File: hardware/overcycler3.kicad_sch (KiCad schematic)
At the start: 133 parts, among them J1 USB_B, J2 AudioJack3_Switch, J3 DIN-5_180degree, J4 AudioJack3_Switch, J5 AudioJack3_Switch, P1 FT232, P2 PANEL, Q1 2SC945, SW1 RESET, SW2 POWER, U1 XT26G02CWSIGA, U2 TL064, U20 AD5328B, U3 LPC1778FBD144, U4 TLV2556, U5 74HC138, U6 TL064, U7 AD5328B, Y1 12MHz

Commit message: hardware: Schematics rework by Guimli
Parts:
- removed C10, C11, C12, C14, C15, C16, C17, C18, C19, C20, C23, C24, C25, C26, C27, C28, C29, C30, C32, C34: 100n, Capacitor_SMD:C_0805_2012Metric, symbol overcycler2-rescue:C
- removed C13: 470u, Capacitor_Tantalum_SMD:CP_EIA-7343-43_Kemet-X, symbol overcycler2-rescue:CP1
- removed C2, C3, C4, C5, C6, C7: 10n, Capacitor_SMD:C_0805_2012Metric, symbol overcycler2-rescue:C
- removed C21, C22, C31: 10u, Capacitor_Tantalum_SMD:CP_EIA-3216-18_Kemet-A, symbol overcycler2-rescue:CP1
- removed J1: USB_B, Connector_USB:USB_B_Lumberg_2411_02_Horizontal, symbol Connector:USB_B
- removed P1: FT232, Connector_PinSocket_2.54mm:PinSocket_1x06_P2.54mm_Vertical, symbol overcycler2-rescue:CONN_6
- removed P2: PANEL, Connector_IDC:IDC-Header_2x20_P2.54mm_Vertical, symbol overcycler2-rescue:CONN_20X2
- removed PS1: IA0505S-2W, JETEKPS:IA0505S-2W, symbol Converter_DCDC:IA0505S
- removed PS2: IB0503LSY-1WR1, JETEKPS:IB0503LSY, symbol Converter_DCDC:IA0503S
- removed R152: 2k7, Resistor_SMD:R_0805_2012Metric, symbol overcycler2-rescue:R
- removed R2, R4: 33, Resistor_SMD:R_0805_2012Metric, symbol overcycler2-rescue:R
- removed R5: 1k5, Resistor_SMD:R_0805_2012Metric, symbol overcycler2-rescue:R
- removed SW2: POWER, SPUN192600:SPUN192600, symbol Switch:SW_Push_DPDT
- added J10: Control_Down, Connector_JST:JST_XH_B7B-XH-A_1x07_P2.50mm_Vertical, symbol Connector_Generic:Conn_01x07
- added J6: Control_Up, Connector_JST:JST_XH_B7B-XH-A_1x07_P2.50mm_Vertical, symbol Connector_Generic:Conn_01x07
- added J7: Keyboard, Connector_JST:JST_XH_B8B-XH-A_1x08_P2.50mm_Vertical, symbol Connector_Generic:Conn_01x08
- added J8: Display, Connector_IDC:IDC-Header_2x08_P2.54mm_Vertical, symbol Connector_Generic:Conn_02x08_Odd_Even
- added J9: FT232, Connector_PinSocket_2.54mm:PinSocket_1x06_P2.54mm_Vertical, symbol Connector_Generic:Conn_01x06
- C1, C112, C113, C114, C35, C37, C38, C39, C40, C41, C42, C43, C44, C45, C46, C47, C50, C51, C8, C9: symbol overcycler2-rescue:C -> Additional:C
- C33, C36, C48, C49: symbol overcycler2-rescue:CP1 -> Additional:CP
- D1, D2, D3, D4, D5: symbol overcycler2-rescue:DIODE -> Additional:DIODE
- OC1: symbol overcycler2-rescue:6N139 -> Isolator:6N139
- R1, R10, R11, R12, R13, R14, R15, R16, R17, R18, R19, R20, R21, R22, R23, R24, R25, R26, R27, R28, R29, R3, R30, R31, R32, R33, R34, R35, R36, R37, R38, R39, R40, R45, R46, R47, R48, R6, R7, R8, R9: symbol overcycler2-rescue:R -> Additional:R
- R151, R41, R42, R43, R44: renamed from R93; symbol overcycler2-rescue:R -> Additional:R
- SW1: symbol overcycler2-rescue:SW_PUSH -> Additional:SW_PUSH
- U1: symbol XT26G02ELGIGA:XT26G02ELGIGA -> Additional:XT26G02ELGIGA
- U2, U6: symbol overcycler2-rescue:TL074 -> Amplifier_Operational:TL064
- U20, U7: symbol AD5328B:AD5328B -> Additional:AD5328B
- U3: symbol LPC1778FBD144:LPC1778FBD144 -> Additional:LPC1778FBD144; Supplier C37701 -> (none)
- U4: symbol overcycler2-rescue:TLV1543 -> Additional:TLV1543
- U5: symbol overcycler2-rescue:74LS138 -> 74xx:74HC138
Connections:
- net +5V: now also U20.1 (~{LDAC}), U7.1 (~{LDAC}), J8.14 (Pin_14); no longer U2.4 (V+), U2.4 (V+), U2.4 (V+), U2.4 (V+), U6.4 (V+), U6.4 (V+), U6.4 (V+), U6.4 (V+)
- net -5V: no longer U2.11 (V-), U2.11 (V-), U2.11 (V-), U2.11 (V-), U6.11 (V-), U6.11 (V-), U6.11 (V-), U6.11 (V-)
- net GND: now also U1.9 (PAD), J10.7 (Pin_7), J6.7 (Pin_7), J8.13 (Pin_13), J9.4 (Pin_4); no longer U20.1 (/LDAC), U7.1 (/LDAC)
- net KP_1_R1: now also J7.1 (Pin_1)
- net KP_2_R2: now also J7.2 (Pin_2)
- net KP_3_R3: now also J7.3 (Pin_3)
- net KP_4_R4: now also J7.4 (Pin_4)
- net KP_5_C1: now also J7.5 (Pin_5)
- net KP_6_C2: now also J7.6 (Pin_6)
- net KP_7_C3: now also J7.7 (Pin_7)
- net KP_8_C4: now also J7.8 (Pin_8)
- net LCD_CTRST: now also R25.1, J8.12 (Pin_12); no longer R25.2, U3.8 (P0[26])
- net LCD_DB4: now also J8.4 (Pin_4)
- net LCD_DB5: now also J8.3 (Pin_3)
- net LCD_DB6: now also J8.2 (Pin_2)
- net LCD_DB7: now also J8.1 (Pin_1)
- net LCD_E1: now also J8.9 (Pin_9)
- net LCD_E2: now also J8.15 (Pin_15)
- net LCD_RS: now also J8.11 (Pin_11)
- net LCD_RW: now also J8.10 (Pin_10)
- net PROG_BOOT: now also J9.6 (Pin_6)
- net PROG_RXD: now also J9.3 (Pin_3)
- net PROG_TXD: now also J9.2 (Pin_2)
- net P_0: now also J6.2 (Pin_2)
- net P_1: now also J6.3 (Pin_3)
- net P_2: now also J6.4 (Pin_4)
- net P_3: now also J6.5 (Pin_5)
- net P_4: now also J6.6 (Pin_6)
- net P_5: now also J10.2 (Pin_2)
- net P_6: now also J10.3 (Pin_3)
- net P_7: now also J10.4 (Pin_4)
- net P_8: now also J10.5 (Pin_5)
- net P_9: now also J10.6 (Pin_6)
- net SPI_SSEL: now also U5.6 (E2); no longer U5.4 (E1)
- net +3.3V renamed +3V3
- net +3V3: now also U5.4 (~{E0}), J10.1 (Pin_1), J6.1 (Pin_1), J9.1 (Pin_1); no longer U5.6 (E3)
- new net: R25.2, U3.8 (P0[26])
- no-connect marks 0 -> 96
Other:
- added sheet Power_Supply (Power_Supply.kicad_sch)
- note removed: "LCD Display is NHD‐0440WH Keypad is 16 keys 4*4 matrix Data entry potentiometers are 4.7k linear taper"
- moved on the sheet: C1, C112, C113, C114, C33, C35, C36, C37, C38, C39, C40, C41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

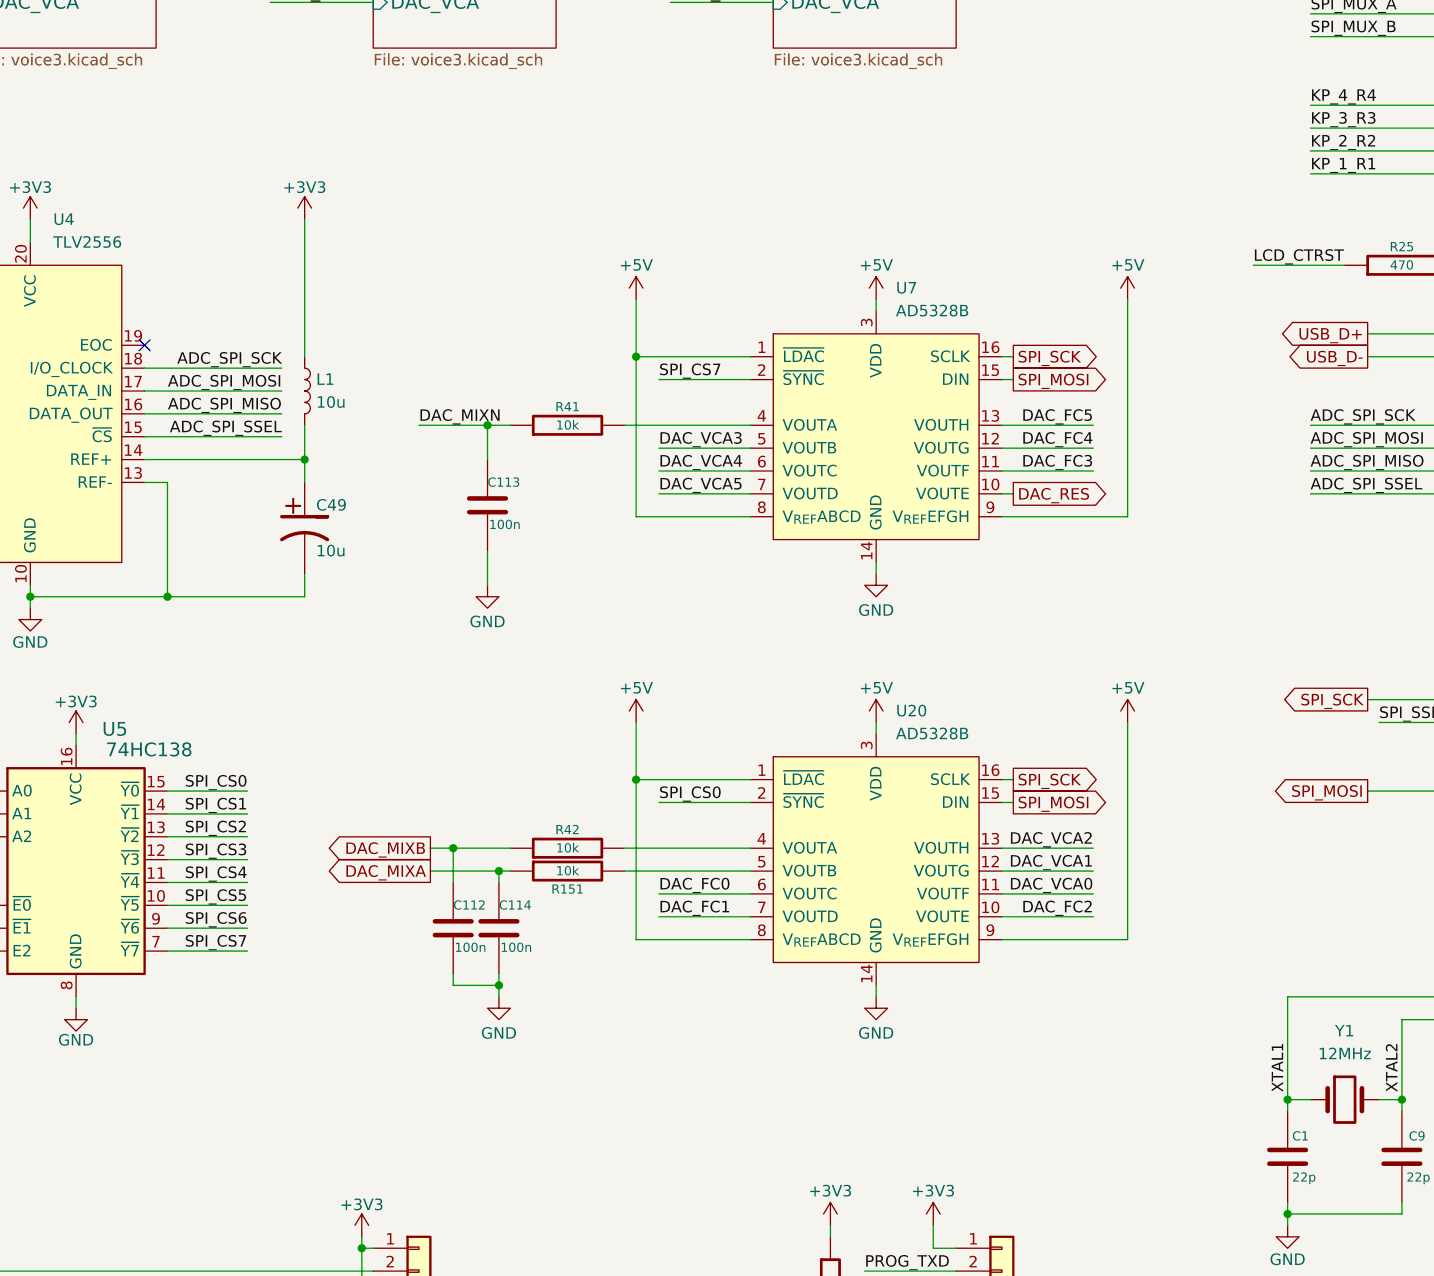
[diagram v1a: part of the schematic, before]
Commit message: hardware: sch update (AD5674R replacing AD5328B*2)
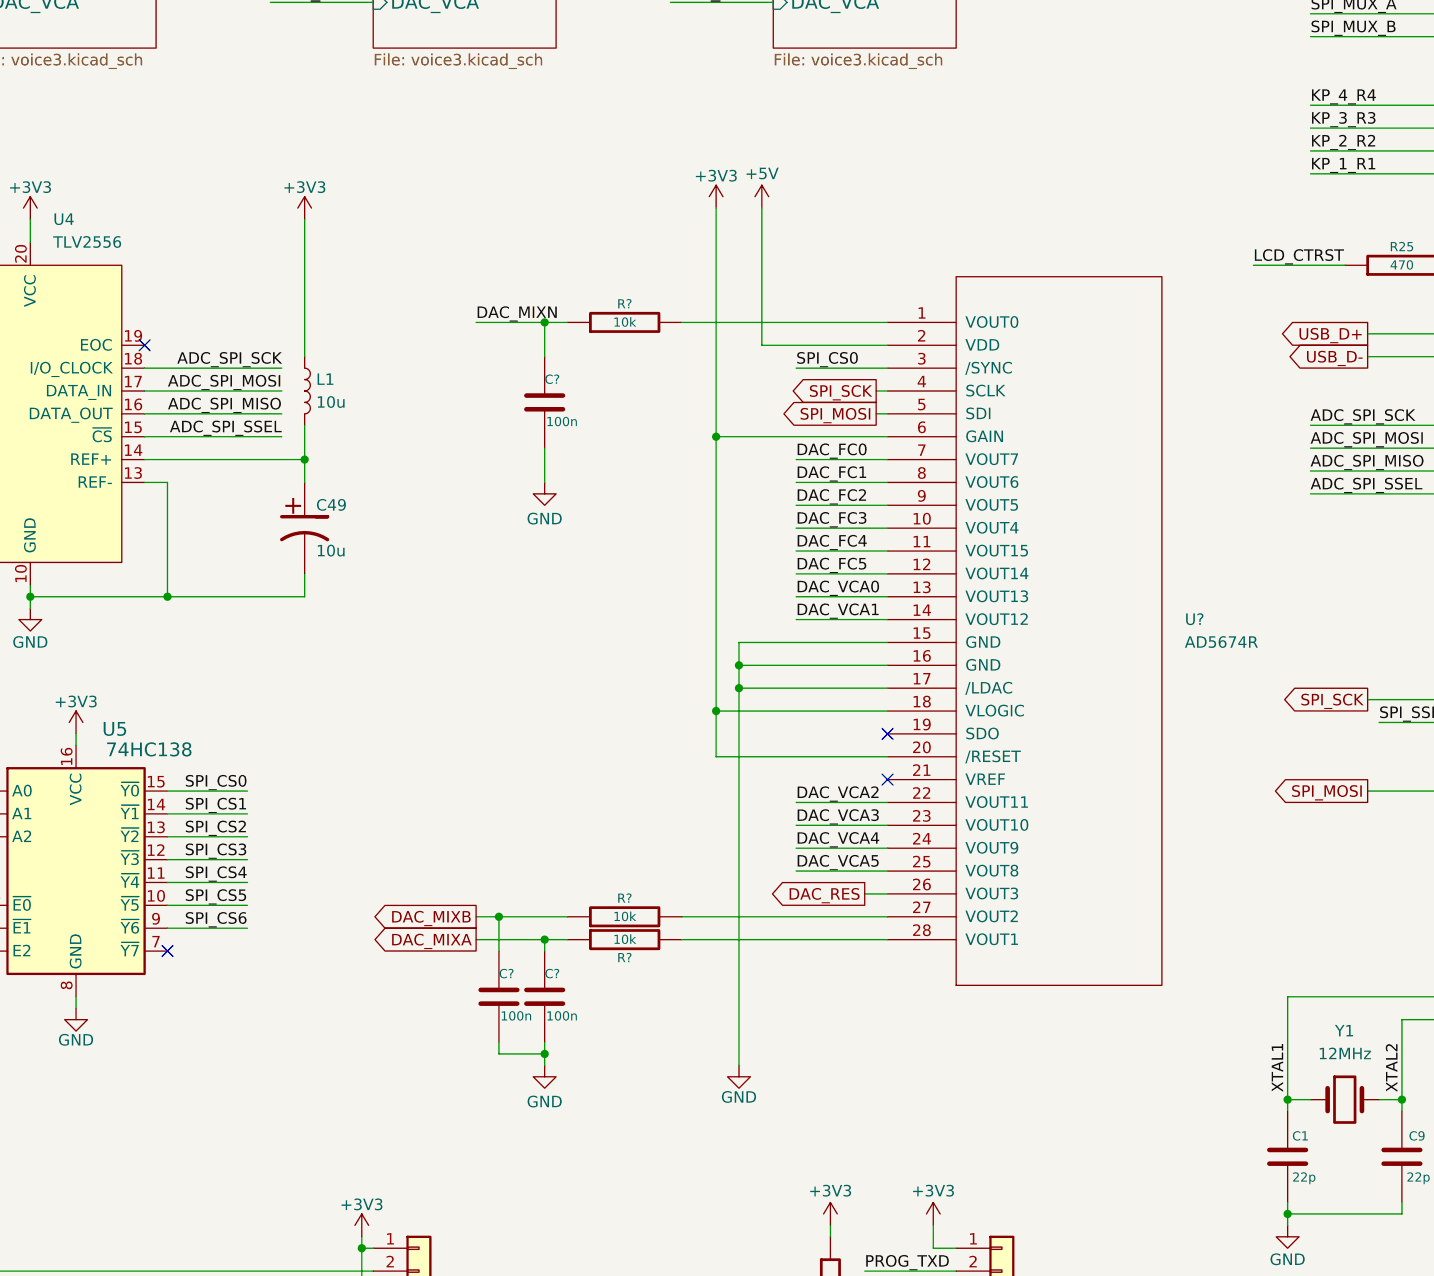
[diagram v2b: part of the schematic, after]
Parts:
- removed C112, C113, C114: 100n, Capacitor_SMD:C_0805_2012Metric, symbol Additional:C
- removed R151, R41, R42: 10k, Resistor_SMD:R_0805_2012Metric, symbol Additional:R
- removed U20, U7: AD5328B, Package_SO:TSSOP-16_4.4x5mm_P0.65mm, symbol Additional:AD5328B
- added C? (x3): 100n, Capacitor_SMD:C_0805_2012Metric, symbol Additional:C
- added R? (x3): 10k, Resistor_SMD:R_0805_2012Metric, symbol Additional:R
- added U?: AD5674R, MODULE, symbol AD5674R:AD5674R
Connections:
- net +3V3: now also U?.18 (VLOGIC), U?.20 (/RESET), U?.6 (GAIN)
- net +5V: now also U?.2 (VDD)
- net DAC_FC0: now also U?.7 (VOUT7)
- net DAC_FC1: now also U?.8 (VOUT6)
- net DAC_FC2: now also U?.9 (VOUT5)
- net DAC_FC3: now also U?.10 (VOUT4)
- net DAC_FC4: now also U?.11 (VOUT15)
- net DAC_FC5: now also U?.12 (VOUT14)
- net DAC_MIXA: now also C?.1, R?.1
- net DAC_MIXB: now also C?.1, R?.1
- net DAC_MIXN: now also C?.1, R?.1
- net DAC_RES: now also U?.26 (VOUT3)
- net DAC_VCA0: now also U?.13 (VOUT13)
- net DAC_VCA1: now also U?.14 (VOUT12)
- net DAC_VCA2: now also U?.22 (VOUT11)
- net DAC_VCA3: now also U?.23 (VOUT10)
- net DAC_VCA4: now also U?.24 (VOUT9)
- net DAC_VCA5: now also U?.25 (VOUT8)
- net GND: now also C?.2, C?.2, C?.2, U?.15 (GND), U?.16 (GND), U?.17 (/LDAC)
- net SPI_CS0: now also U?.3 (/SYNC)
- net SPI_MOSI: now also U?.5 (SDI)
- net SPI_SCK: now also U?.4 (SCLK)
- net SPI_CS7: no longer names the net of U5.7 (~{Y7})
- new net: R?.2, U?.1 (VOUT0)
- new net: R?.2, U?.27 (VOUT2)
- new net: R?.2, U?.28 (VOUT1)
- no-connect marks 96 -> 99
